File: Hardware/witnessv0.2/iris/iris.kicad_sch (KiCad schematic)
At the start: 10 parts

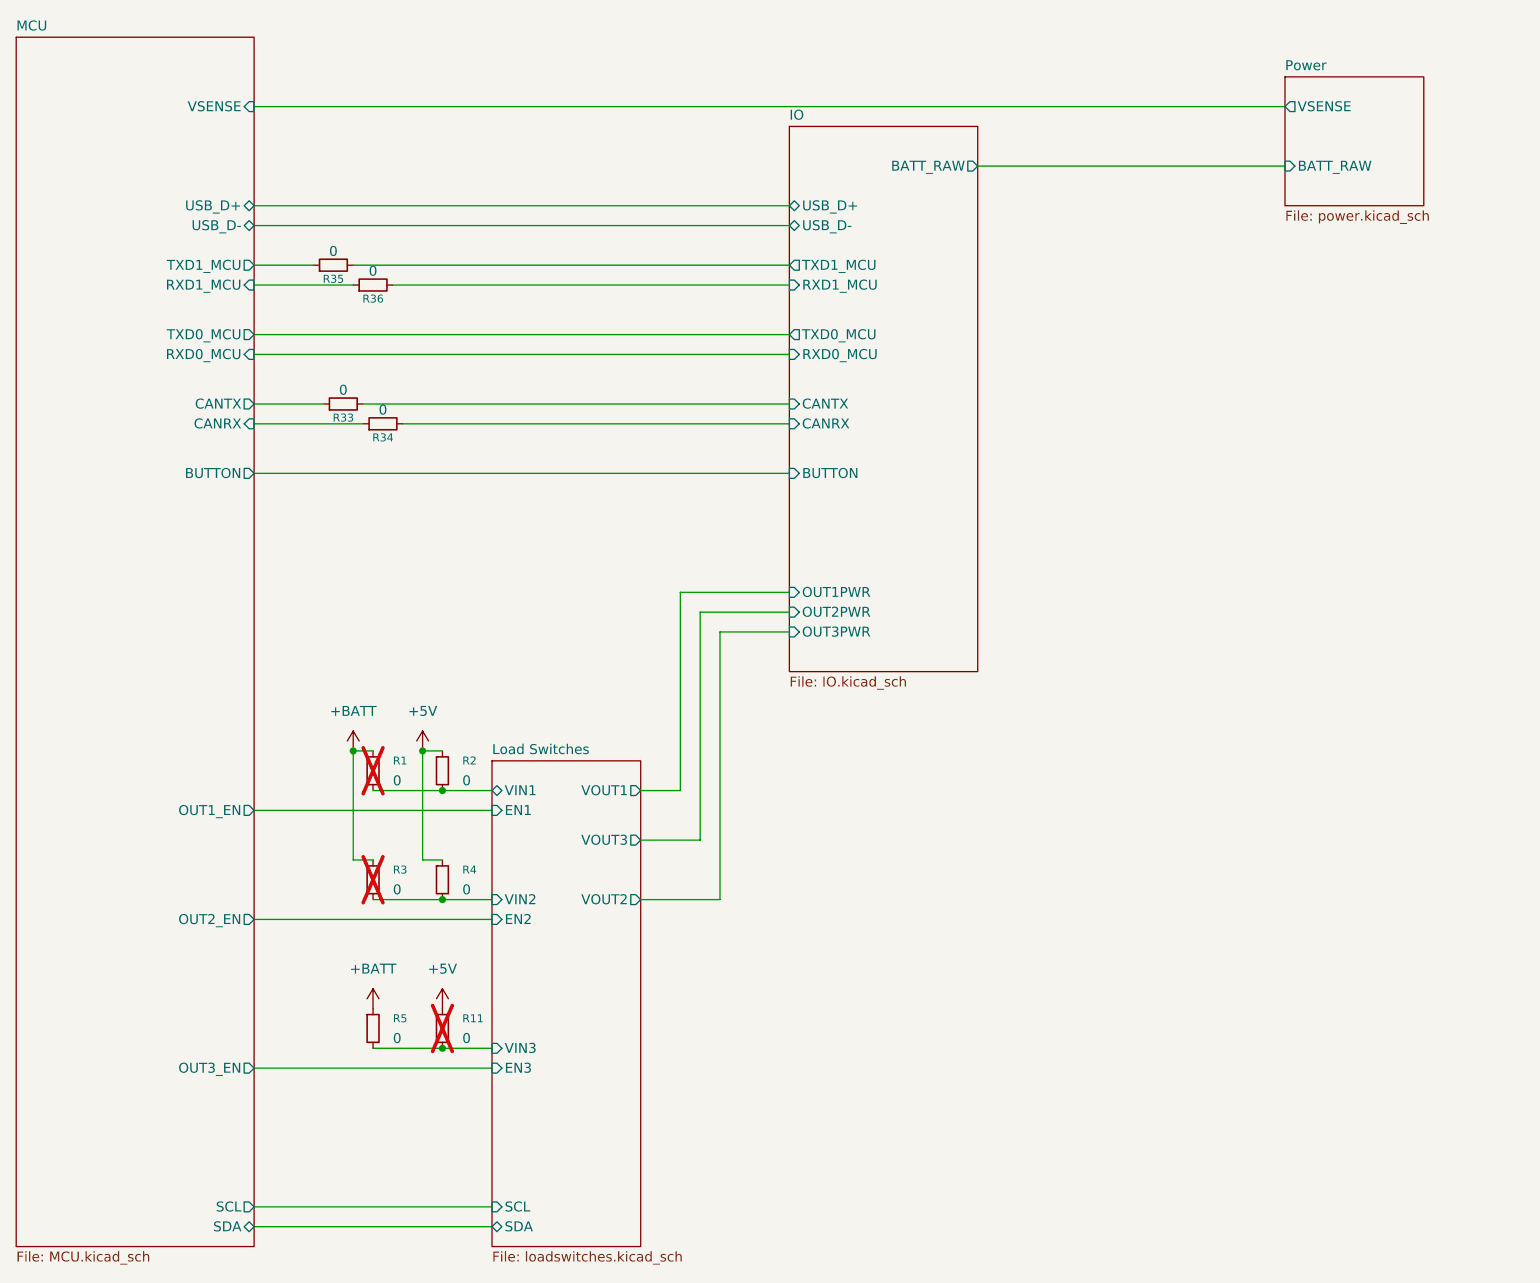
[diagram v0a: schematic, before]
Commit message: iris inital layout
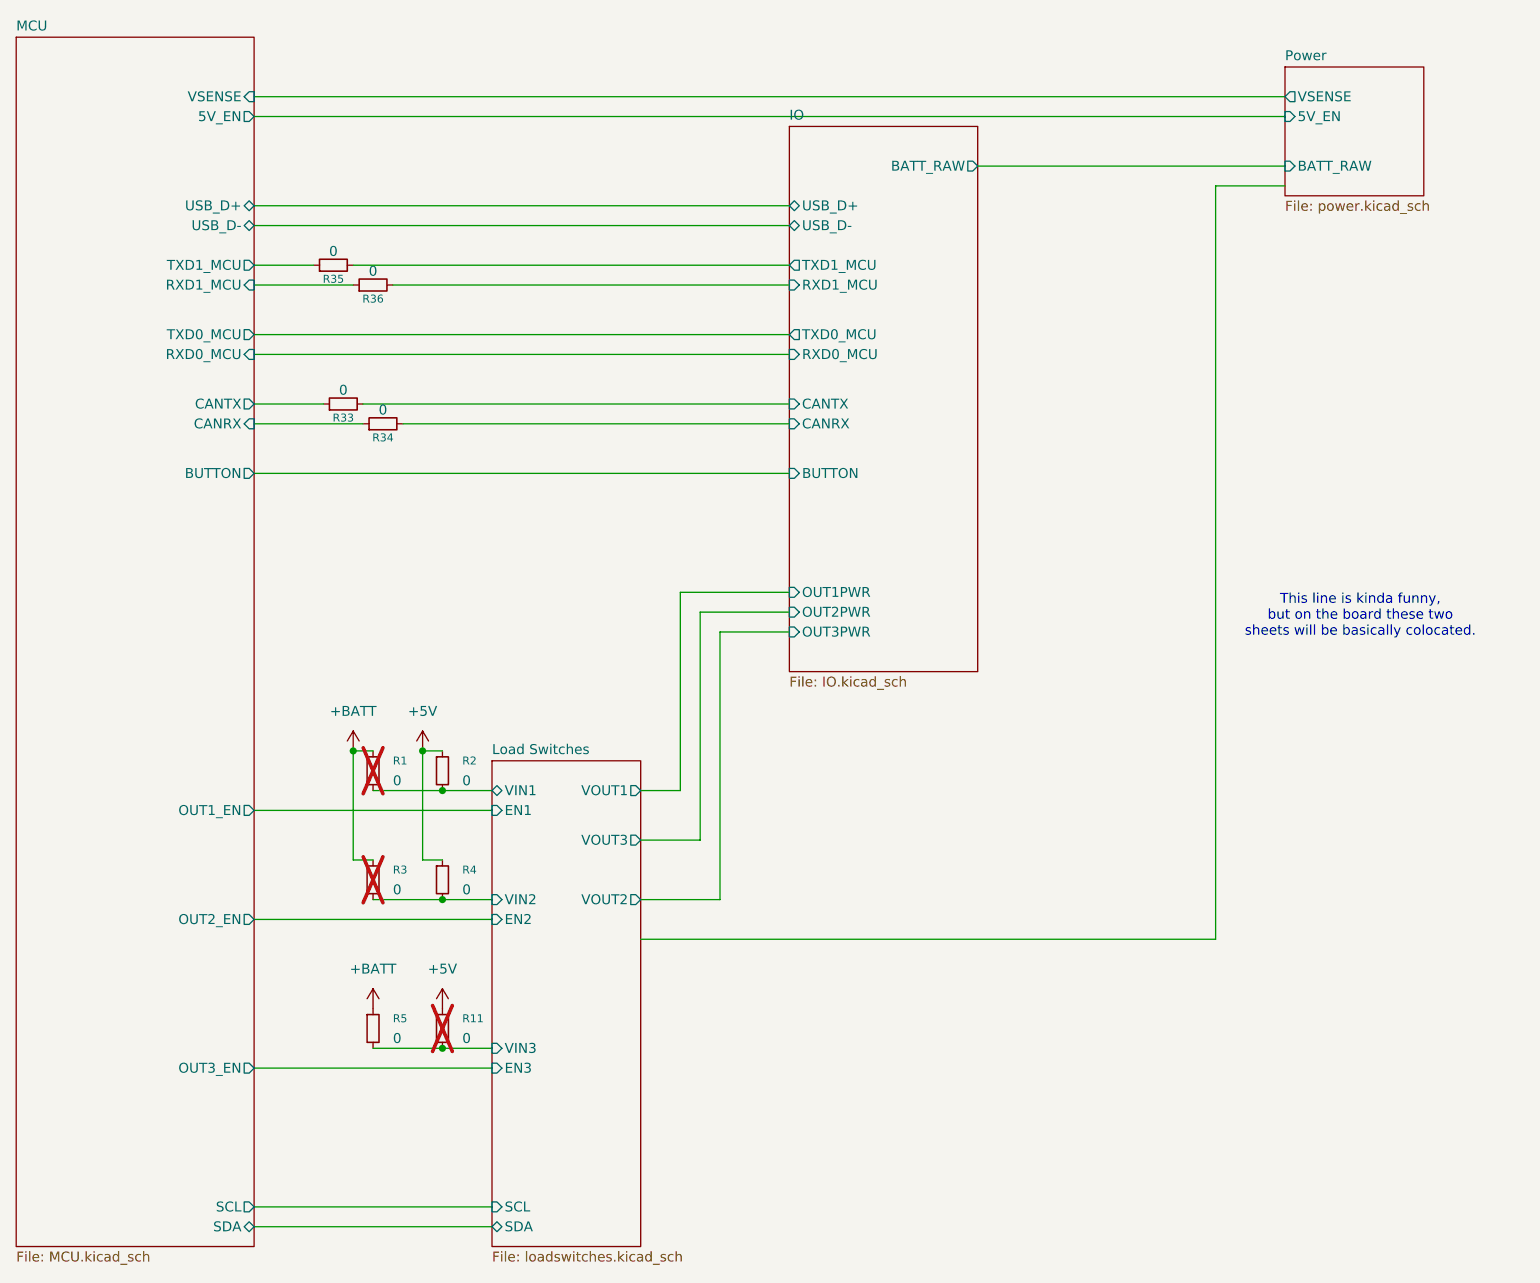
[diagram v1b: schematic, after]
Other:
- sheet MCU ports: added 5V_EN; removed none
- sheet Power ports: added 5V_EN; removed none
- note added: "This line is kinda funny, but on the board these two sheets will be basically colocated."
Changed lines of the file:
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@@
 		(company "WITNESS")
+	)
+	(text "This line is kinda funny, \nbut on the board these two \nsheets will be basically colocated."
+		(exclude_from_sim no)
+		(at 226.822 98.298 0)
+		(effects
+			(font
+				(size 1.27 1.27)
+			)
+		)
 	)
 	(junction
@@
 	(wire
 		(pts
+			(xy 208.28 139.7) (xy 208.28 43.18)
+		)
+		(stroke
+			(width 0)
+			(type default)
+		)
+	)
+	(wire
+		(pts
 			(xy 85.09 123.19) (xy 115.57 123.19)
 		)
@@
 	(wire
 		(pts
+			(xy 139.7 120.65) (xy 139.7 95.25)
+		)
+		(stroke
+			(width 0)
+			(type default)
+		)
+	)
+	(wire
+		(pts
+			(xy 97.79 53.34) (xy 153.67 53.34)
+		)
+		(stroke
+			(width 0)
+			(type default)
+		)
+	)
+	(wire
+		(pts
+			(xy 85.09 45.72) (xy 153.67 45.72)
+		)
+		(stroke
+			(width 0)
+			(type default)
+		)
+	)
+	(wire
+		(pts
+			(xy 144.78 100.33) (xy 153.67 100.33)
+		)
+		(stroke
+			(width 0)
+			(type default)
+		)
+	)
+	(wire
+		(pts
+			(xy 115.57 156.21) (xy 85.09 156.21)
+		)
+		(stroke
+			(width 0)
+			(type default)
+		)
+	)
+	(wire
+		(pts
+			(xy 100.33 120.65) (xy 109.22 120.65)
+		)
+		(stroke
+			(width 0)
+			(type default)
+		)
+	)
+	(wire
+		(pts
+			(xy 85.09 48.26) (xy 153.67 48.26)
+		)
+		(stroke
+			(width 0)
+			(type default)
+		)
+	)
+	(wire
+		(pts
+			(xy 134.62 139.7) (xy 208.28 139.7)
+		)
+		(stroke
+			(width 0)
+			(type default)
+		)
+	)
+	(wire
+		(pts
+			(xy 139.7 95.25) (xy 153.67 95.25)
+		)
+		(stroke
+			(width 0)
+			(type default)
+		)
+	)
+	(wire
+		(pts
+			(xy 85.09 31.75) (xy 217.17 31.75)
+		)
+		(stroke
+			(width 0)
+			(type default)
+		)
+	)
+	(wire
+		(pts
+			(xy 106.68 129.54) (xy 109.22 129.54)
+		)
+		(stroke
+			(width 0)
+			(type default)
+		)
+	)
+	(wire
+		(pts
+			(xy 85.09 64.77) (xy 153.67 64.77)
+		)
+		(stroke
+			(width 0)
+			(type default)
+		)
+	)
+	(wire
+		(pts
+			(xy 106.68 115.57) (xy 109.22 115.57)
+		)
+		(stroke
+			(width 0)
+			(type default)
+		)
+	)
+	(wire
+		(pts
+			(xy 115.57 137.16) (xy 85.09 137.16)
+		)
+		(stroke
+			(width 0)
+			(type default)
+		)
+	)
+	(wire
+		(pts
+			(xy 85.09 176.53) (xy 115.57 176.53)
+		)
+		(stroke
+			(width 0)
+			(type default)
+		)
+	)
+	(wire
+		(pts
+			(xy 99.06 71.12) (xy 153.67 71.12)
+		)
+		(stroke
+			(width 0)
+			(type default)
+		)
+	)
+	(wire
+		(pts
+			(xy 134.62 134.62) (xy 144.78 134.62)
+		)
+		(stroke
+			(width 0)
+			(type default)
+		)
+	)
+	(wire
+		(pts
+			(xy 134.62 120.65) (xy 139.7 120.65)
+		)
+		(stroke
+			(width 0)
+			(type default)
+		)
+	)
+	(wire
+		(pts
+			(xy 97.79 115.57) (xy 100.33 115.57)
+		)
+		(stroke
+			(width 0)
+			(type default)
+		)
+	)
+	(wire
+		(pts
 			(xy 177.8 40.64) (xy 217.17 40.64)
 		)
@@
 	(wire
 		(pts
-			(xy 139.7 120.65) (xy 139.7 95.25)
-		)
-		(stroke
-			(width 0)
-			(type default)
-		)
-	)
-	(wire
-		(pts
-			(xy 97.79 53.34) (xy 153.67 53.34)
-		)
-		(stroke
-			(width 0)
-			(type default)
-		)
-	)
-	(wire
-		(pts
-			(xy 85.09 45.72) (xy 153.67 45.72)
-		)
-		(stroke
-			(width 0)
-			(type default)
-		)
-	)
-	(wire
-		(pts
-			(xy 144.78 100.33) (xy 153.67 100.33)
-		)
-		(stroke
-			(width 0)
-			(type default)
-		)
-	)
-	(wire
-		(pts
-			(xy 115.57 156.21) (xy 85.09 156.21)
-		)
-		(stroke
-			(width 0)
-			(type default)
-		)
-	)
-	(wire
-		(pts
-			(xy 100.33 120.65) (xy 109.22 120.65)
-		)
-		(stroke
-			(width 0)
-			(type default)
-		)
-	)
-	(wire
-		(pts
-			(xy 85.09 48.26) (xy 153.67 48.26)
-		)
-		(stroke
-			(width 0)
-			(type default)
-		)
-	)
-	(wire
-		(pts
-			(xy 139.7 95.25) (xy 153.67 95.25)
-		)
-		(stroke
-			(width 0)
-			(type default)
-		)
-	)
-	(wire
-		(pts
-			(xy 106.68 129.54) (xy 109.22 129.54)
-		)
-		(stroke
-			(width 0)
-			(type default)
-		)
-	)
-	(wire
-		(pts
-			(xy 85.09 64.77) (xy 153.67 64.77)
-		)
-		(stroke
-			(width 0)
-			(type default)
-		)
-	)
-	(wire
-		(pts
-			(xy 106.68 115.57) (xy 109.22 115.57)
-		)
-		(stroke
-			(width 0)
-			(type default)
-		)
-	)
-	(wire
-		(pts
-			(xy 115.57 137.16) (xy 85.09 137.16)
-		)
-		(stroke
-			(width 0)
-			(type default)
-		)
-	)
-	(wire
-		(pts
-			(xy 85.09 176.53) (xy 115.57 176.53)
-		)
-		(stroke
-			(width 0)
-			(type default)
-		)
-	)
-	(wire
-		(pts
-			(xy 99.06 71.12) (xy 153.67 71.12)
-		)
-		(stroke
-			(width 0)
-			(type default)
-		)
-	)
-	(wire
-		(pts
-			(xy 134.62 134.62) (xy 144.78 134.62)
-		)
-		(stroke
-			(width 0)
-			(type default)
-		)
-	)
-	(wire
-		(pts
-			(xy 134.62 120.65) (xy 139.7 120.65)
-		)
-		(stroke
-			(width 0)
-			(type default)
-		)
-	)
-	(wire
-		(pts
-			(xy 97.79 115.57) (xy 100.33 115.57)
-		)
-		(stroke
-			(width 0)
-			(type default)
-		)
-	)
-	(wire
-		(pts
 			(xy 85.09 173.99) (xy 115.57 173.99)
 		)
@@
 	(wire
 		(pts
+			(xy 85.09 34.29) (xy 217.17 34.29)
+		)
+		(stroke
+			(width 0)
+			(type default)
+		)
+	)
+	(wire
+		(pts
 			(xy 85.09 53.34) (xy 92.71 53.34)
 		)
@@
 	(wire
 		(pts
-			(xy 85.09 33.02) (xy 217.17 33.02)
-		)
-		(stroke
-			(width 0)
-			(type default)
-		)
-	)
-	(wire
-		(pts
 			(xy 109.22 134.62) (xy 115.57 134.62)
 		)
@@
 		(pts
 			(xy 104.14 73.66) (xy 153.67 73.66)
+		)
+		(stroke
+			(width 0)
+			(type default)
+		)
+	)
+	(wire
+		(pts
+			(xy 208.28 43.18) (xy 217.17 43.18)
 		)
 		(stroke
@@
 		)
 		(pin "VSENSE" input
-			(at 85.09 33.02 0)
+			(at 85.09 31.75 0)
 			(effects
 				(font
@@
 		(pin "BUTTON" output
 			(at 85.09 80.01 0)
+			(effects
+				(font
+					(size 1.27 1.27)
+				)
+				(justify right)
+			)
+		)
+		(pin "5V_EN" output
+			(at 85.09 34.29 0)
 			(effects
 				(font
@@
 	)
 	(sheet
-		(at 217.17 29.21)
+		(at 217.17 27.94)
 		(size 17.78 16.51)
 		(exclude_from_sim no)
@@
 		)
 		(property "Sheetname" "Power"
-			(at 217.17 28.4984 0)
+			(at 217.17 27.2284 0)
 			(show_name no)
 			(do_not_autoplace no)
@@
 		)
 		(property "Sheetfile" "power.kicad_sch"
-			(at 217.17 46.3046 0)
+			(at 217.17 45.0346 0)
 			(show_name no)
 			(do_not_autoplace no)
@@
 		)
 		(pin "VSENSE" output
-			(at 217.17 33.02 180)
+			(at 217.17 31.75 180)
 			(effects
 				(font
@@
 			(effects
 				(font
+					(size 1.27 1.27)
+				)
+				(justify left)
+			)
+		)
+		(pin "5V_EN" input
+			(at 217.17 34.29 180)
+			(effects
+				(font
